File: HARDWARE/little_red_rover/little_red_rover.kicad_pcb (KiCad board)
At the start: 2 copper layers, 127.3 x 82.2 mm, 38 parts, among them J1 USB_C_Receptacle_USB2.0_14P, J2 Conn_01x04_Socket, J3 Conn_01x02_Socket, J4 Conn_01x02_Socket, U1 ESP32-C3-MINI-1, U2 BQ24230RGT, U3 MIC5504-3.3YM5, U4 MIC2876-5.0YMT-TR, U5 DRV8212P, U6 DRV8212P, U7 GP1S094HCZ0F, U8 GP1S094HCZ0F

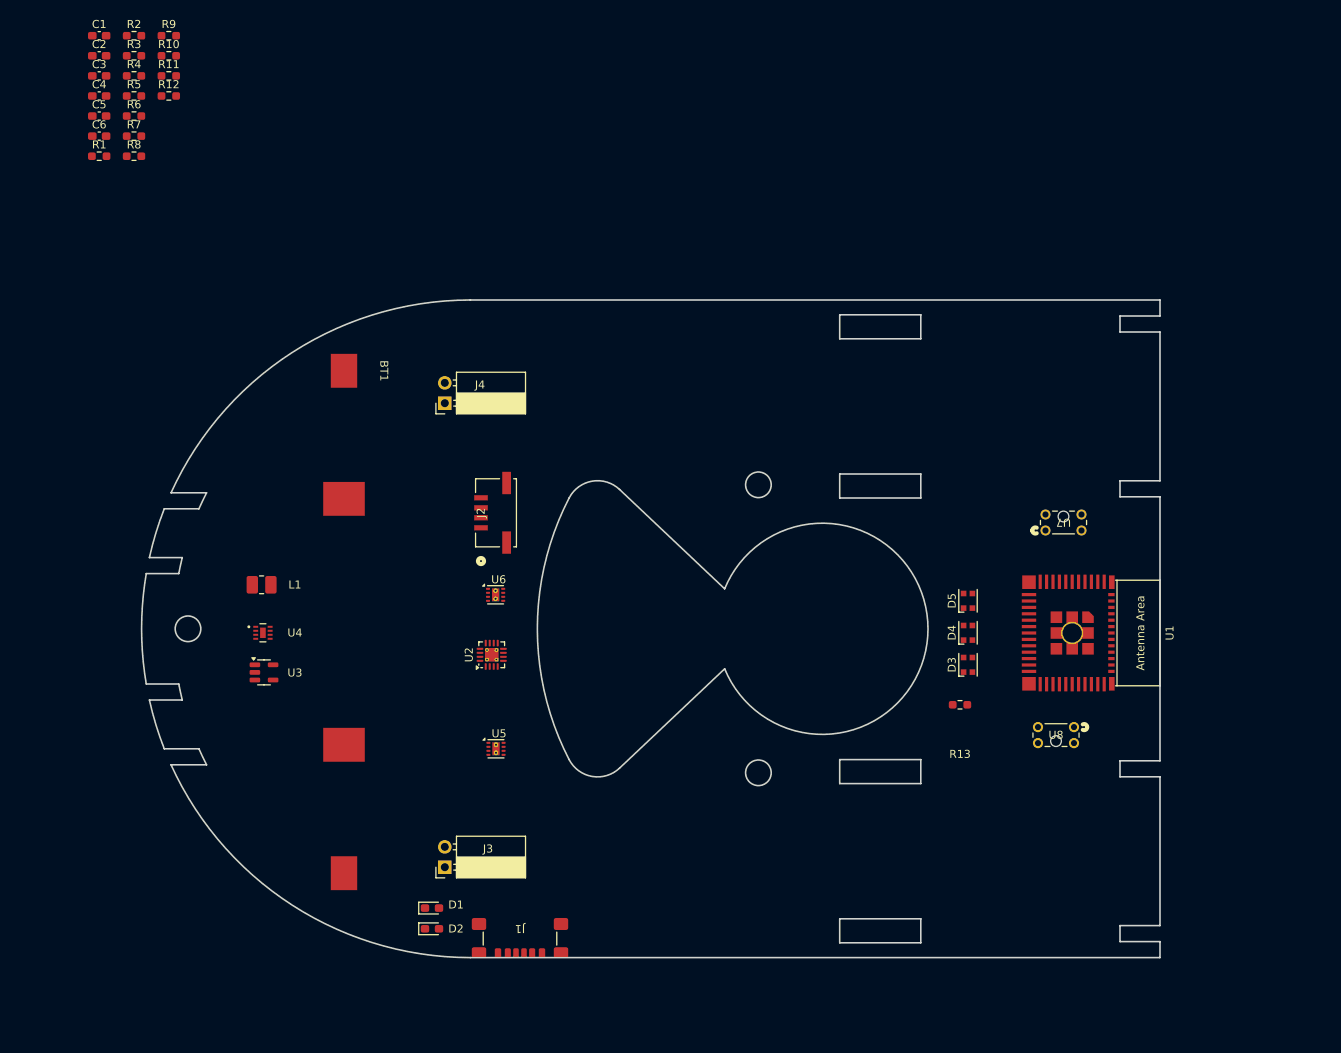
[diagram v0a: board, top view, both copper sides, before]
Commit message: v1.0 board layout
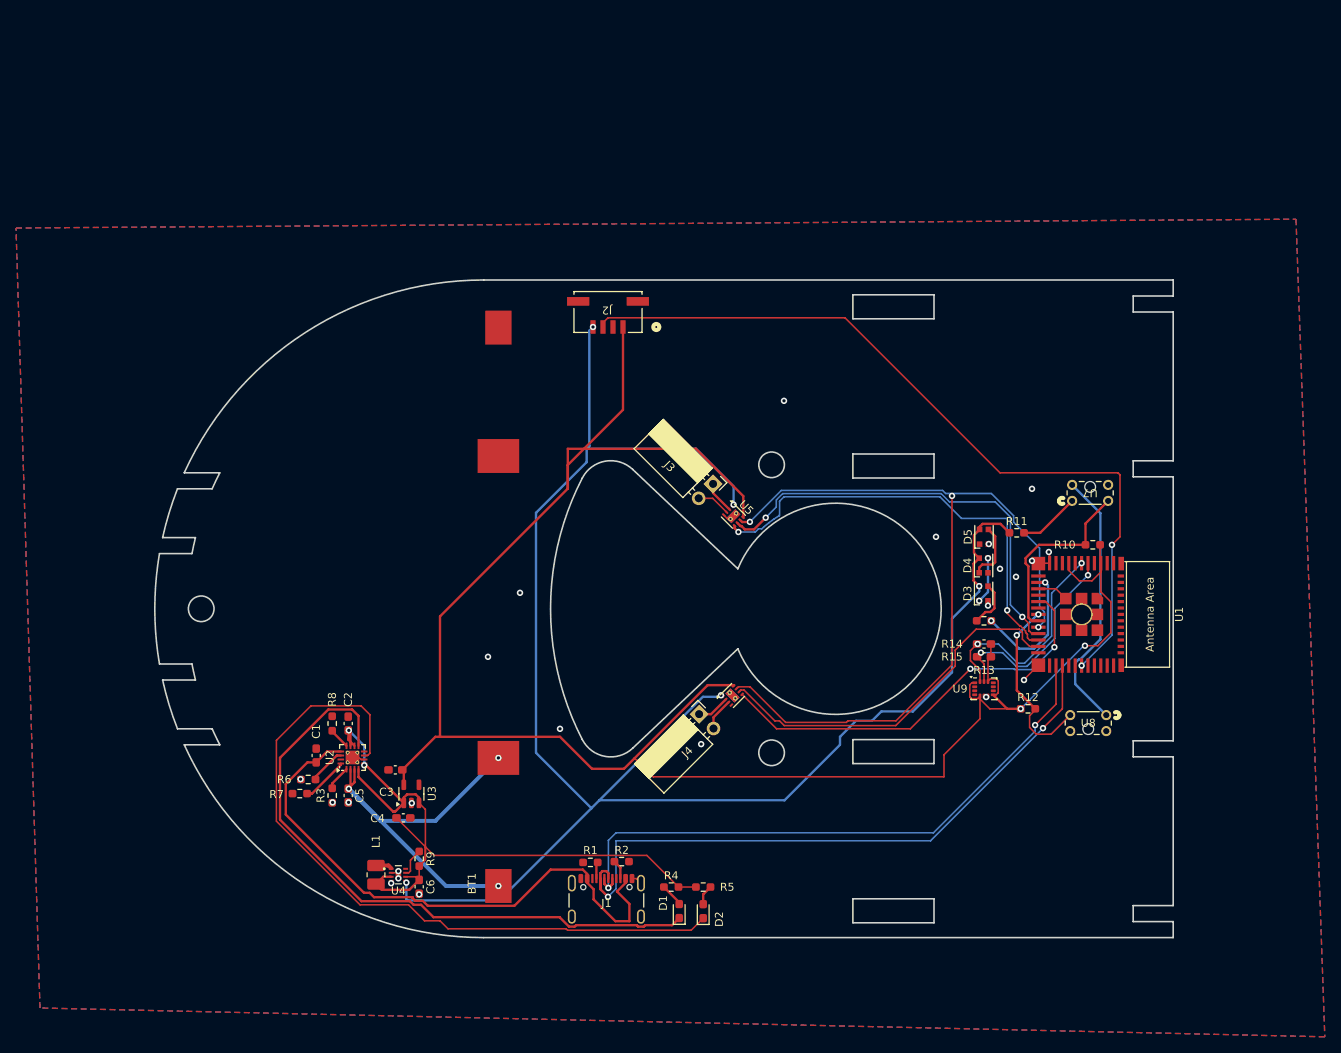
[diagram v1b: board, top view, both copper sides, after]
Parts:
- added R14: 10k, Capacitor_SMD:C_0603_1608Metric_Pad1.08x0.95mm_HandSolder, F.Cu at (190.0, 104.4)
- added R15: 10k, Capacitor_SMD:C_0603_1608Metric_Pad1.08x0.95mm_HandSolder, F.Cu at (190.0, 106.0)
- added U9: LSM6DS3, Package_LGA:LGA-14_3x2.5mm_P0.5mm_LayoutBorder3x4y, F.Cu at (190.0, 110.0)
- J1: footprint Connector_USB:USB_C_Receptacle_GCT_USB4135-GF-A_6P_TopMnt_Horizontal -> Connector_USB:USB_C_Receptacle_GCT_USB4105-xx-A_16P_TopMnt_Horizontal
- moved R12 131.9 mm to (195.5, 112.5)
- moved R10 130.7 mm to (203.6, 92.0), turned to 180 degrees
- moved R5 121.8 mm to (154.9, 134.8), turned to 180 degrees
- moved R4 121.6 mm to (150.9, 134.8)
- moved R11 120.4 mm to (194.1, 90.5)
- moved R2 119.9 mm to (144.7, 131.6)
- moved R9 107.5 mm to (119.4, 131.2), turned to -90 degrees
- moved R1 107.5 mm to (140.8, 131.7), turned to 180 degrees
- moved C6 102.0 mm to (119.4, 134.7), turned to -90 degrees
- moved C4 97.9 mm to (117.4, 126.1)
- moved R3 95.7 mm to (108.5, 123.3), turned to 90 degrees
- moved C3 94.3 mm to (116.4, 120.1), turned to 180 degrees
- moved C1 94.0 mm to (106.5, 118.3), turned to 90 degrees
- moved C5 90.5 mm to (110.5, 123.3), turned to -90 degrees
- moved C2 89.1 mm to (110.5, 114.3), turned to 90 degrees
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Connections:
- C1 pad 1: +5V -> /usb_5v
- J1 pad A9: +5V -> /usb_5v
- J1 pad B9: +5V -> /usb_5v
- U1 pad 5: unconnected-(U1-GPIO2/ADC1_CH2-Pad5) -> /imu_scl
- U1 pad 6: unconnected-(U1-GPIO3/ADC1_CH3-Pad6) -> /imu_sda
- U2 pad 13: +5V -> /usb_5v
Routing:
- net +3.3V: track 0.00 -> 251.1 mm, vias 0 -> 2
- net +5V: track 0.00 -> 217.3 mm, vias 0 -> 5
- net /motor_sleep: track 0.00 -> 106.0 mm, vias 0 -> 3
- net /lidar_tx: track 0.00 -> 98.8 mm, vias 0 -> 2
- net /charger_out: track 0.00 -> 91.8 mm, vias 0 -> 2
- net Net-(D2-K): track 0.00 -> 89.3 mm
- net /usb_data_+: track 0.00 -> 81.9 mm, vias 0 -> 2
- net Net-(D1-K): track 0.00 -> 80.1 mm
- net /usb_data_-: track 0.00 -> 77.5 mm, vias 0 -> 2
- net /usb_5v: track 0.00 -> 72.5 mm
- net /left_motor_pwm_b: track 0.00 -> 55.9 mm, vias 0 -> 2
- net /left_motor_pwm_a: track 0.00 -> 54.6 mm, vias 0 -> 2
- net /right_motor_pwm_b: track 0.00 -> 52.2 mm, vias 0 -> 2
- net Net-(BT1-+): track 0.00 -> 52.1 mm, vias 0 -> 3
- net /right_motor_pwm_a: track 0.00 -> 46.9 mm
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- added copper zone on B.Cu, net GND
- added copper zone on F.Cu, net GND
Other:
- board text added: "little red rover v1.0"
